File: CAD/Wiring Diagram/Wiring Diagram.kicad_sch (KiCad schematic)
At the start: 13 parts, among them M1 Motor_Servo, M2 Motor_Servo, M3 Motor_Servo, M4 Motor_Servo, M5 Motor_Servo, M6 Motor_Servo, U1 ESP32-DEVKITC, U2 TCS3200, U3 TCS3200, U4 TCS3200, U5 TCS3200, U6 TCS3200, U7 TCS3200

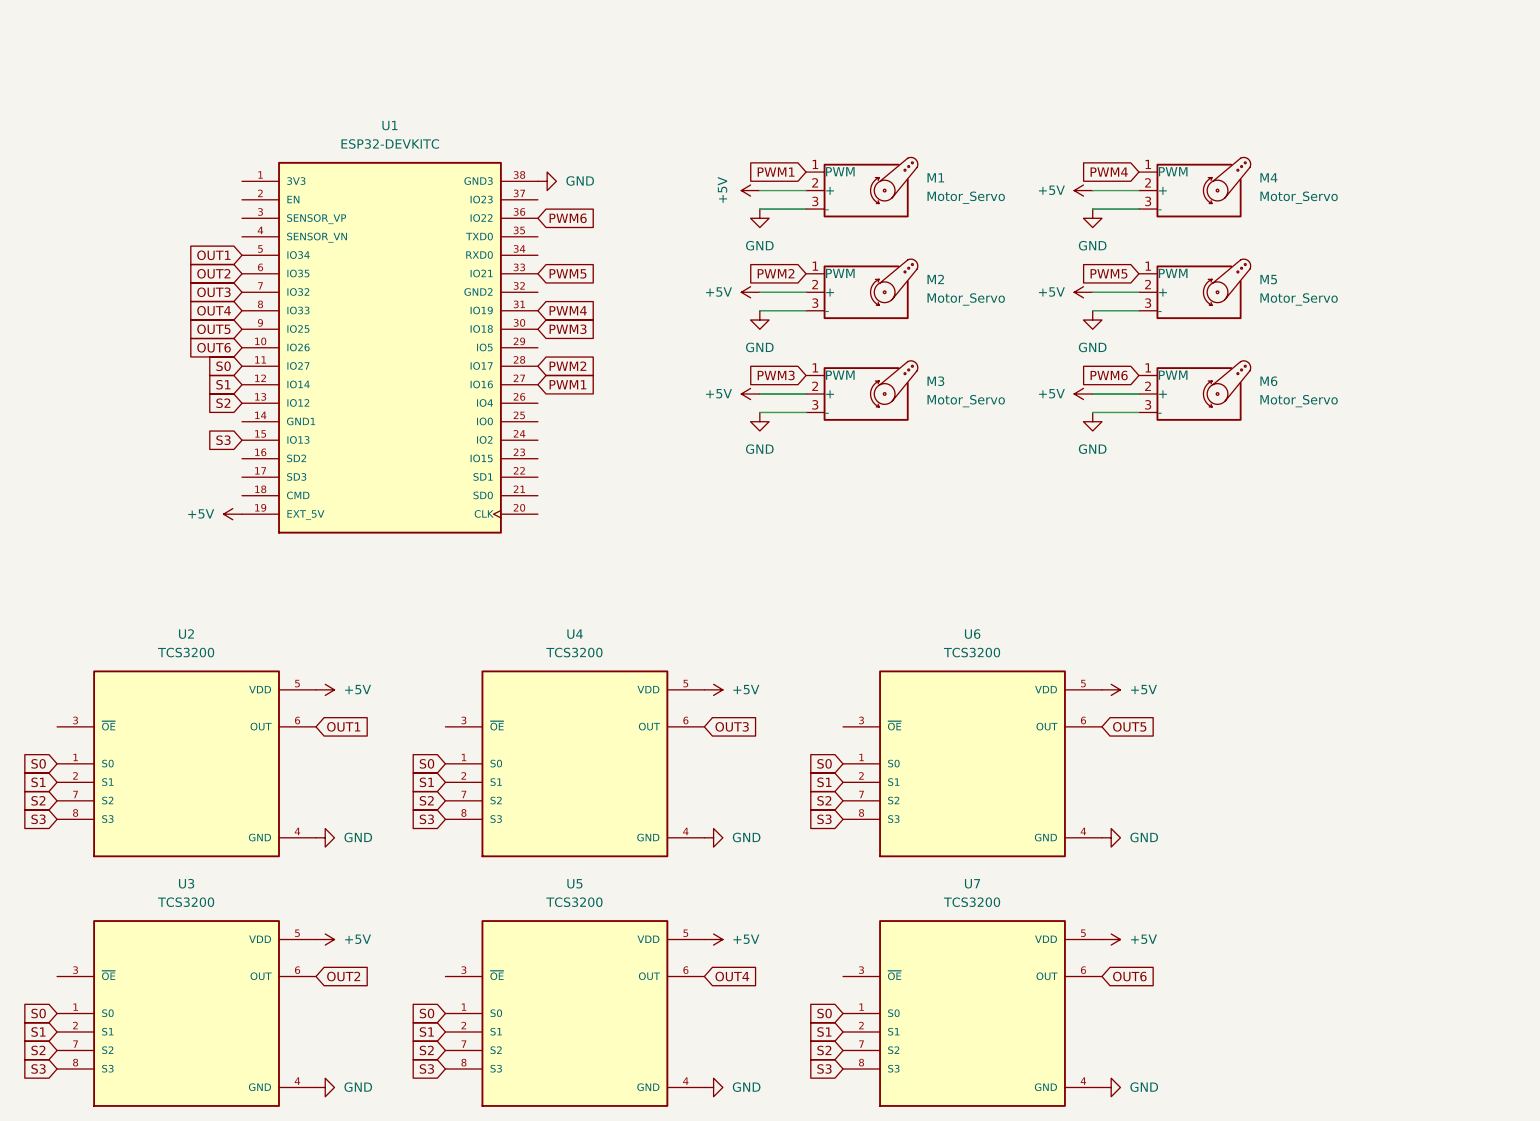
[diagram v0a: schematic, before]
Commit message: Yesterday + Today
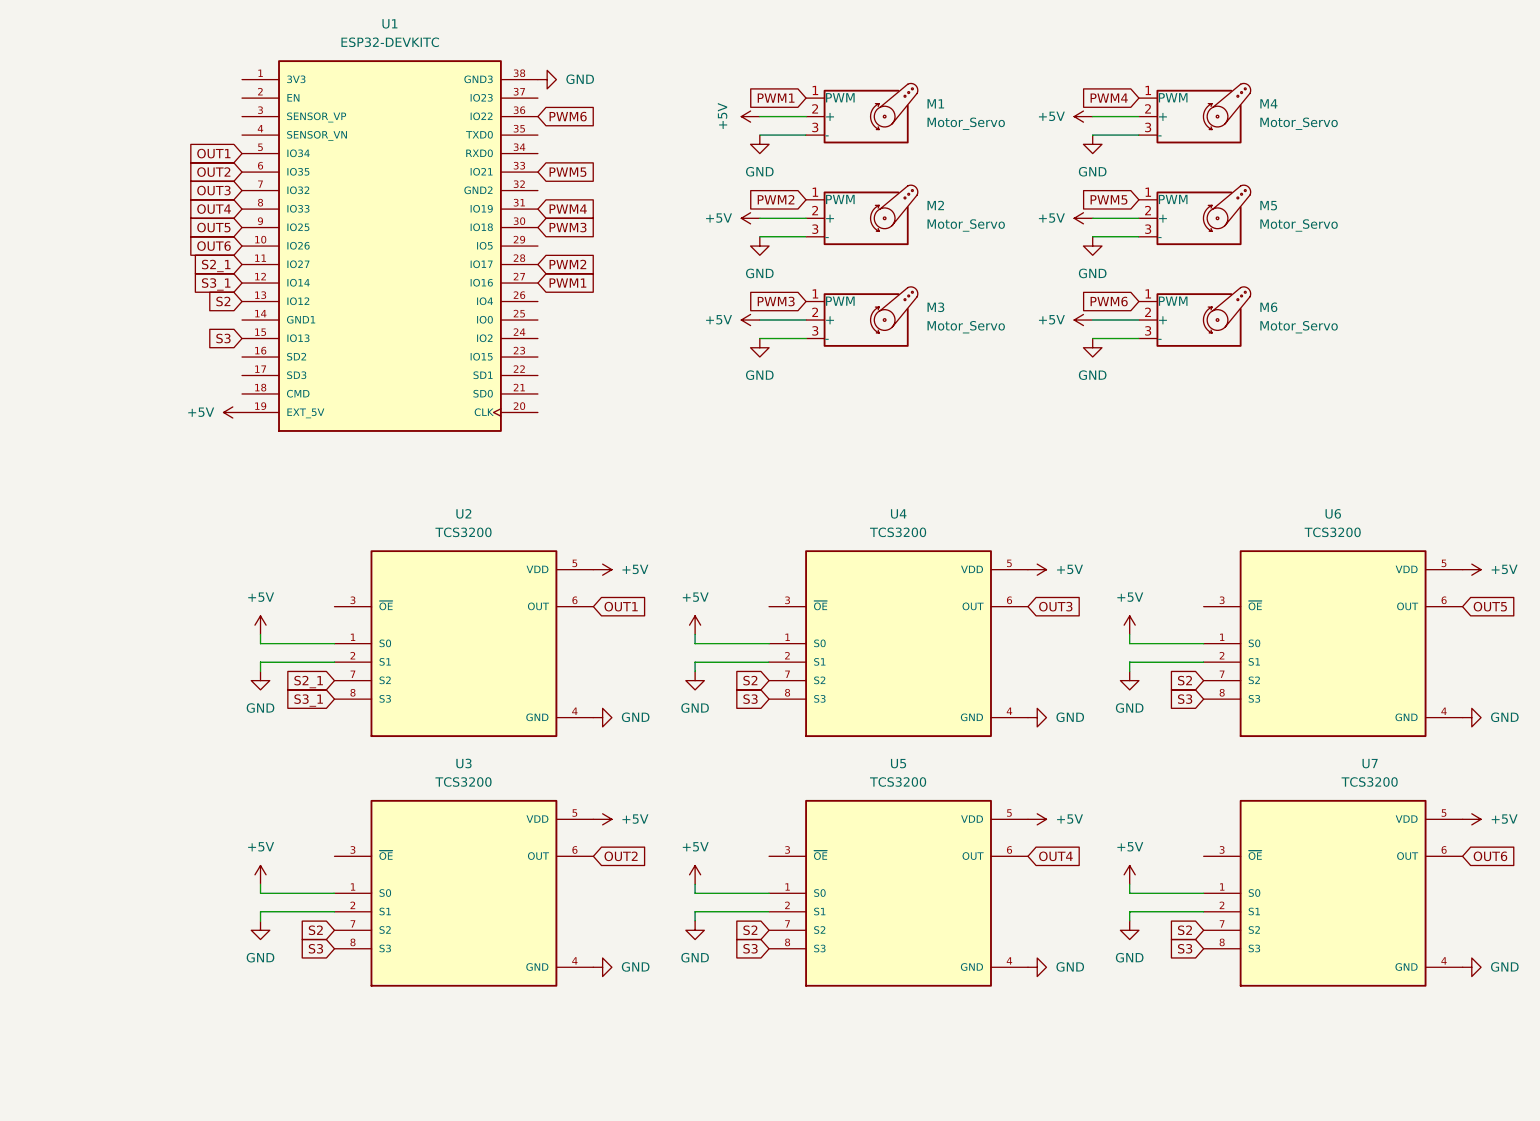
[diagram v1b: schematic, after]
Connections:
- net +5V: now also U2.1 (S0), U3.1 (S0), U4.1 (S0), U5.1 (S0), U6.1 (S0), U7.1 (S0)
- net GND: now also U2.2 (S1), U3.2 (S1), U4.2 (S1), U5.2 (S1), U6.2 (S1), U7.2 (S1)
- net S2: no longer U2.7 (S2)
- net S3: no longer U2.8 (S3)
- removed net S0: U1.11 (IO27), U2.1 (S0), U3.1 (S0), U4.1 (S0), U5.1 (S0), U6.1 (S0), U7.1 (S0)
- removed net S1: U1.12 (IO14), U2.2 (S1), U3.2 (S1), U4.2 (S1), U5.2 (S1), U6.2 (S1), U7.2 (S1)
- new net S2_1: U1.11 (IO27), U2.7 (S2)
- new net S3_1: U1.12 (IO14), U2.8 (S3)
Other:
- moved on the sheet: M1, M2, M3, M4, M5, M6, U1, U2, U3, U4, U5, U6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
